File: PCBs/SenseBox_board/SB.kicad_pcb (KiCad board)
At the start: 2 copper layers, 73.7 x 78.7 mm, 13 parts, among them J1 Jack-DC, J2 Conn_01x20, J3 Conn_01x20, J7 Conn_01x08_Female, J9 Conn_01x08_Female

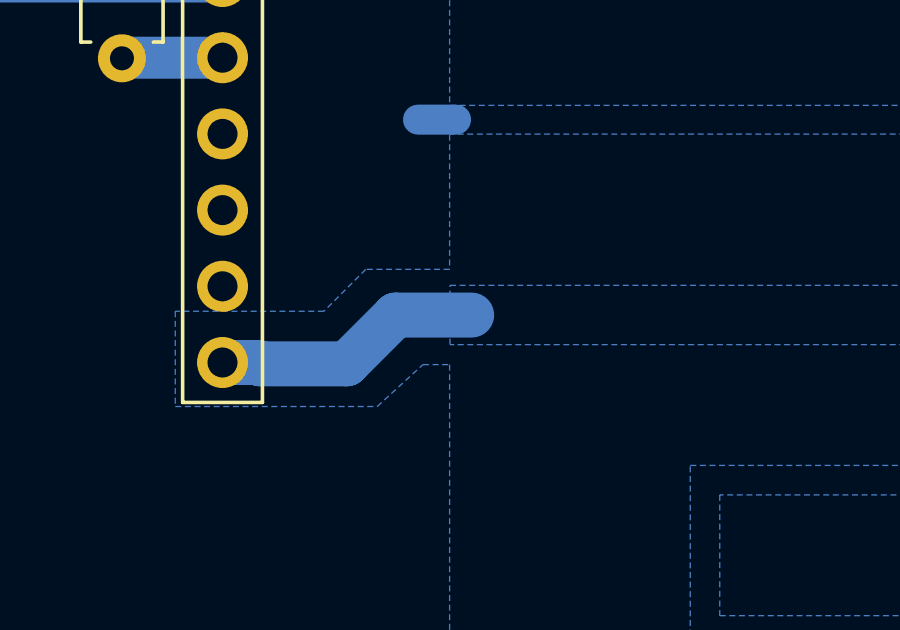
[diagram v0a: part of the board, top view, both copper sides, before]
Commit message: added gerbers
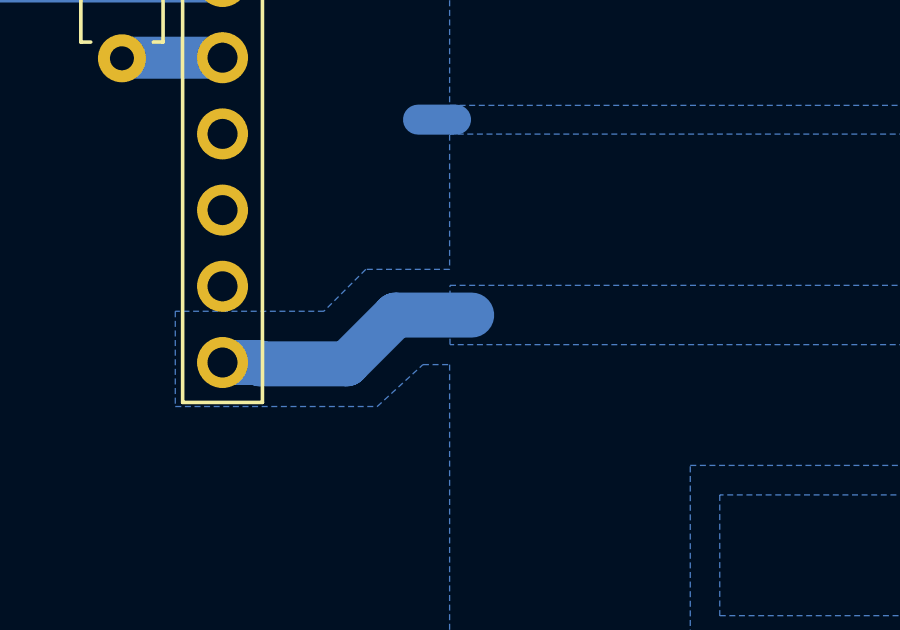
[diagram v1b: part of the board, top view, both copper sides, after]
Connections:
- J9 pad 8: Net-(J9-Pad8) -> /GND
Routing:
- net Net-(J9-Pad8): track 9.00 -> 0.00 mm
- net /GND: track 111.9 -> 120.9 mm
- removed copper zone on B.Cu, net (none)
